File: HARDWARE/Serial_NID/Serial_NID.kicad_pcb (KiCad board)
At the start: 2 copper layers, 40 x 20.3 mm, 14 parts, among them J1 CONN_01X04, J2 CONN_01X07, J3 USB_OTG, U1 TPS2550, U2 STM32L011Gx, U3 FT230XQ

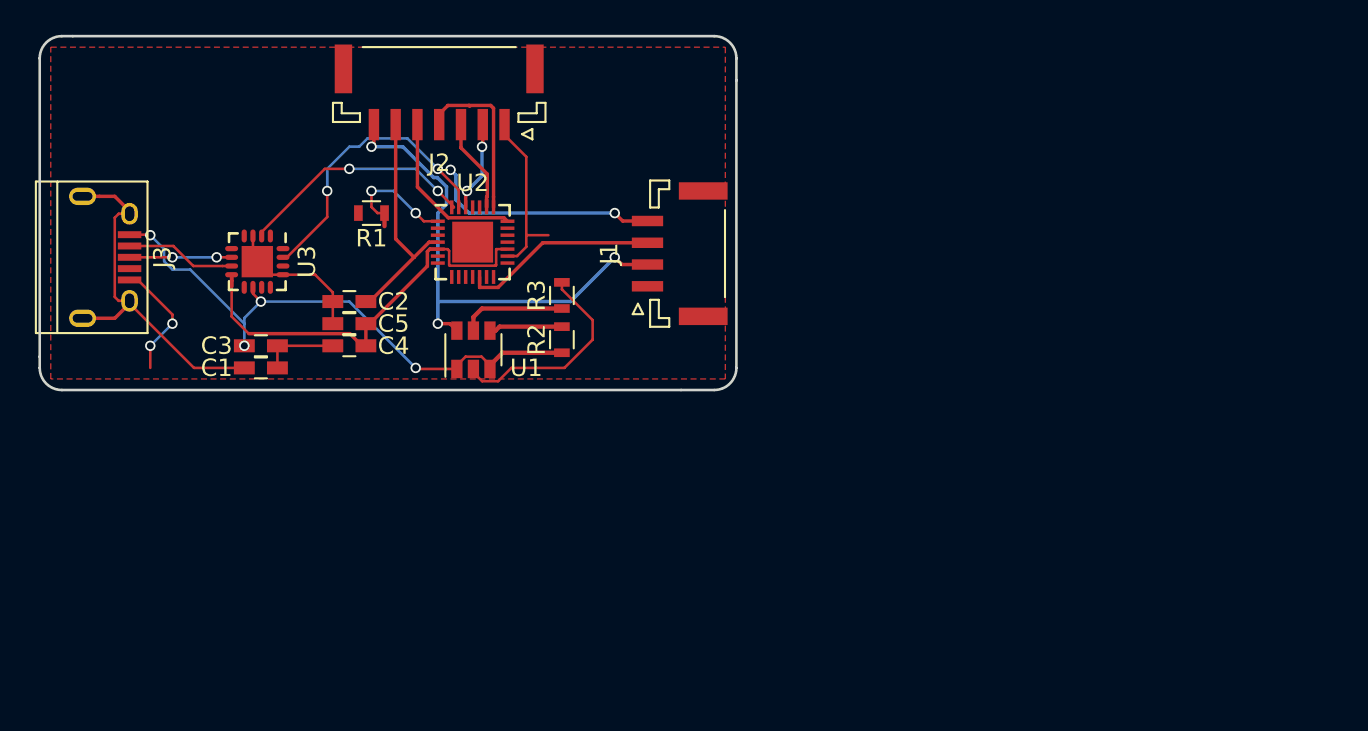
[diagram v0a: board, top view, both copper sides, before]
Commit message: updated pcb
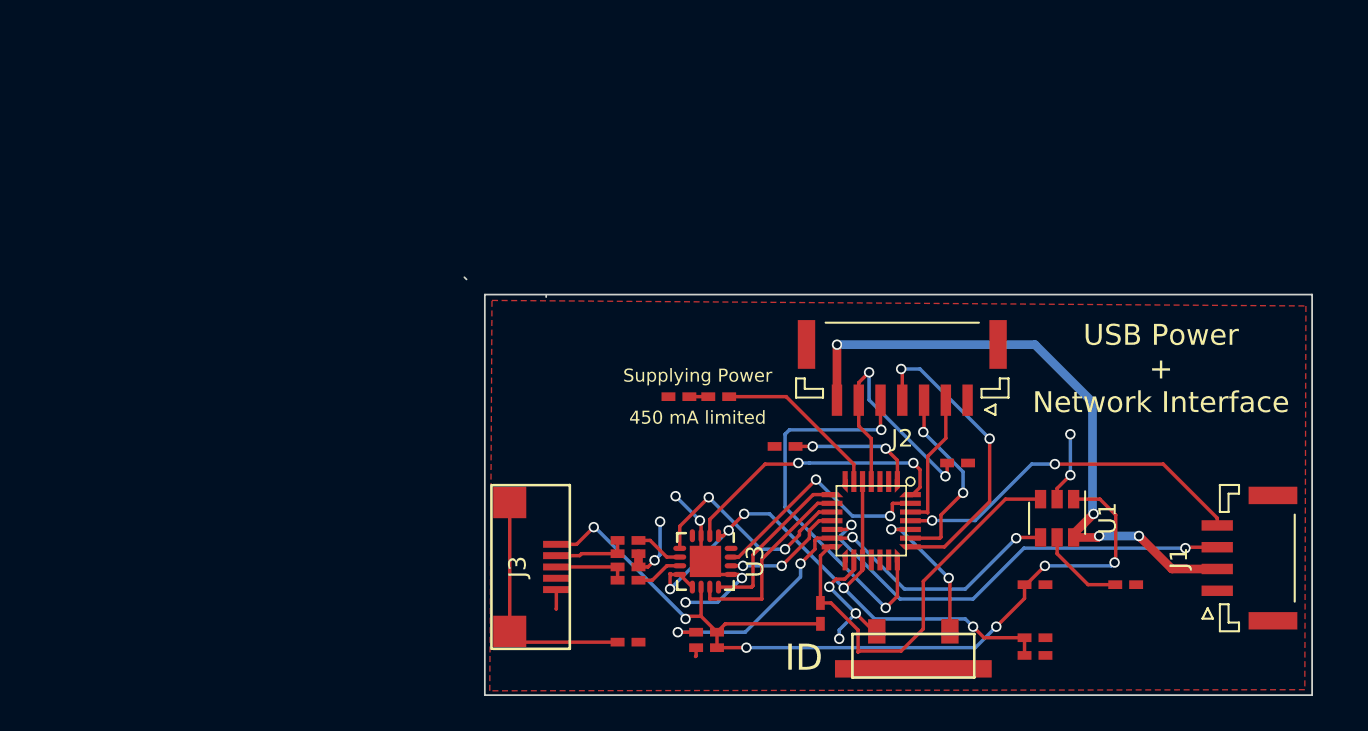
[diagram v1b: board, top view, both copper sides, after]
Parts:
- added C6: C, ZF_footprints:ZF_SMD_NonPol_0402_cap, F.Cu at (125.2, 104.1)
- added C7: C, ZF_footprints:ZF_SMD_NonPol_0402_cap, F.Cu at (125.2, 103.4)
- added C8: C, ZF_footprints:ZF_SMD_NonPol_0402_cap, F.Cu at (148.6, 105.2)
- added D1: LED, ZF_footprints:ZF_SMD_NonPol_0402, F.Cu at (128.1, 94.4)
- added R4: R, ZF_footprints:ZF_SMD_NonPol_0402, F.Cu at (125.2, 104.9)
- added R5: R, ZF_footprints:ZF_SMD_NonPol_0402, F.Cu at (125.2, 102.6)
- added R6: R, ZF_footprints:ZF_SMD_NonPol_0402, F.Cu at (136.3, 106.8)
- added R7: R, ZF_footprints:ZF_SMD_NonPol_0402, F.Cu at (130.4, 94.4)
- added SW1: SW_PUSH, ZF_footprints:ZF_SW_Momentary_SideMtg, F.Cu at (141.6, 110.5)
- C1, C2, C3, C4, C5: footprint Capacitors_SMD:C_0603_HandSoldering -> ZF_footprints:ZF_SMD_NonPol_0402_cap
- J3: footprint Connectors:USB_Micro-B -> ZF_footprints:JW_USBMICROB_SMT
- R1, R2, R3: footprint Resistors_SMD:R_0603 -> ZF_footprints:ZF_SMD_NonPol_0402
- U2: footprint Housings_DFN_QFN:UQFN-28-1EP_4x4mm_Pitch0.4mm -> ZF_footprints:ZF_IC_UFQFPN28-050
- moved C5 43.3 mm to (148.6, 108.2), turned to 0 degrees
- moved C4 43.2 mm to (148.6, 109.2), turned to 0 degrees
- moved J1 37.1 mm to (160.7, 103.6)
- moved R3 36.4 mm to (153.8, 105.2), turned to 0 degrees
- moved C2 36.1 mm to (144.1, 98.2), turned to 0 degrees
- moved U1 34.9 mm to (149.9, 101.3), turned to 270 degrees
- moved U3 31.0 mm to (129.7, 103.8)
- moved J2 30.9 mm to (141.0, 93.0)
- moved C1 30.9 mm to (129.7, 108.8), turned to 0 degrees
- moved J3 30.0 mm to (119.4, 104.1)
- moved U2 27.9 mm to (139.2, 101.5), turned to 180 degrees
- moved R1 27.3 mm to (134.2, 97.2)
- moved C3 26.3 mm to (125.2, 108.5)
- moved R2 18.7 mm to (129.7, 107.9), turned to 180 degrees
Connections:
- J3 pad 2: Net-(J3-Pad2) -> Net-(C7-Pad1)
- J3 pad 3: Net-(J3-Pad3) -> Net-(C6-Pad2)
- U1 pad 3: +5V -> EN
- U2 pad 10: Net-(U2-Pad10) -> CBUS2
- U2 pad 11: Net-(U2-Pad11) -> CBUS3
- U2 pad 13: Net-(U2-Pad13) -> FAULT
- U2 pad 14: Net-(U2-Pad14) -> EN
- U2 pad 6: Net-(U2-Pad6) -> LED1
- U2 pad 8: Net-(U2-Pad8) -> CBUS0
- U2 pad 9: Net-(U2-Pad9) -> CBUS1
- U3 pad 1: Net-(U3-Pad1) -> +3V3
- U3 pad 11: Net-(U3-Pad11) -> CBUS1
- U3 pad 12: Net-(U3-Pad12) -> CBUS0
- U3 pad 14: Net-(U3-Pad14) -> CBUS3
- U3 pad 5: Net-(U3-Pad5) -> CBUS2
- U3 pad 6: Net-(J3-Pad3) -> Net-(R5-Pad1)
- U3 pad 7: Net-(J3-Pad2) -> Net-(R4-Pad1)
- U3 pad 9: Net-(U3-Pad9) -> +3V3
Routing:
- net EN: track 0.00 -> 23.2 mm
- net FAULT: track 4.23 -> 27.4 mm, vias 0 -> 4
- net +5V: track 33.3 -> 52.0 mm, vias 4 -> 6
- net GND: track 43.7 -> 27.8 mm, vias 2 -> 11
- net A1IN: track 11.3 -> 26.6 mm, vias 0 -> 2
- net SWDIO: track 9.57 -> 22.6 mm, vias 0 -> 2
- net CBUS2: track 0.00 -> 12.9 mm, vias 0 -> 2
- net CBUS1: track 0.00 -> 11.3 mm
- net +3V3: track 25.7 -> 35.9 mm, vias 0 -> 5
- net LED1: track 0.00 -> 9.76 mm
- net CBUS0: track 0.00 -> 9.61 mm
- net SWITCH: track 0.00 -> 8.66 mm, vias 0 -> 2
- net SWCLK: track 9.74 -> 17.6 mm, vias 0 -> 2
- net +5VD: track 29.2 -> 36.6 mm, vias 3 -> 4
- net A1EX: track 13.4 -> 20.7 mm
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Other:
- board size 40 x 20.3 mm -> 48.7 x 24 mm
- net class Default: trace_width 0.15 -> 0.2
- net class POWEr added: clearance 0.1, trace_width 0.5, via_dia 0.6, via_drill 0.4
- rule pad_to_mask_clearance: 0.2 -> 0
- rule trace_min: 0.1 -> 0.2
- board text added: "ID"
- board text added: "Supplying Power 450 mA limited"
- board text added: "USB Power + Network Interface"
